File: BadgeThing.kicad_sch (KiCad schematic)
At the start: 62 parts, among them J2 Ext 5V, J3 External 3V3, J4 SWD Header, J5 USB_C_Receptacle_USB2.0, J6 Connector_Generic_Conn_01x02, J7 Conn_01x06, SW1 ESP RESET, SW2 Left, SW3 Down, SW4 Select, SW5 Up, SW6 Right, SW7 BOOTSEL, U1 ESP-12F, U3 RP2040, U4 NCP1117-3.3_SOT223, U5 W25Q32JVSS, U6 USBLC6-2SC6, Y1 12.000MHz

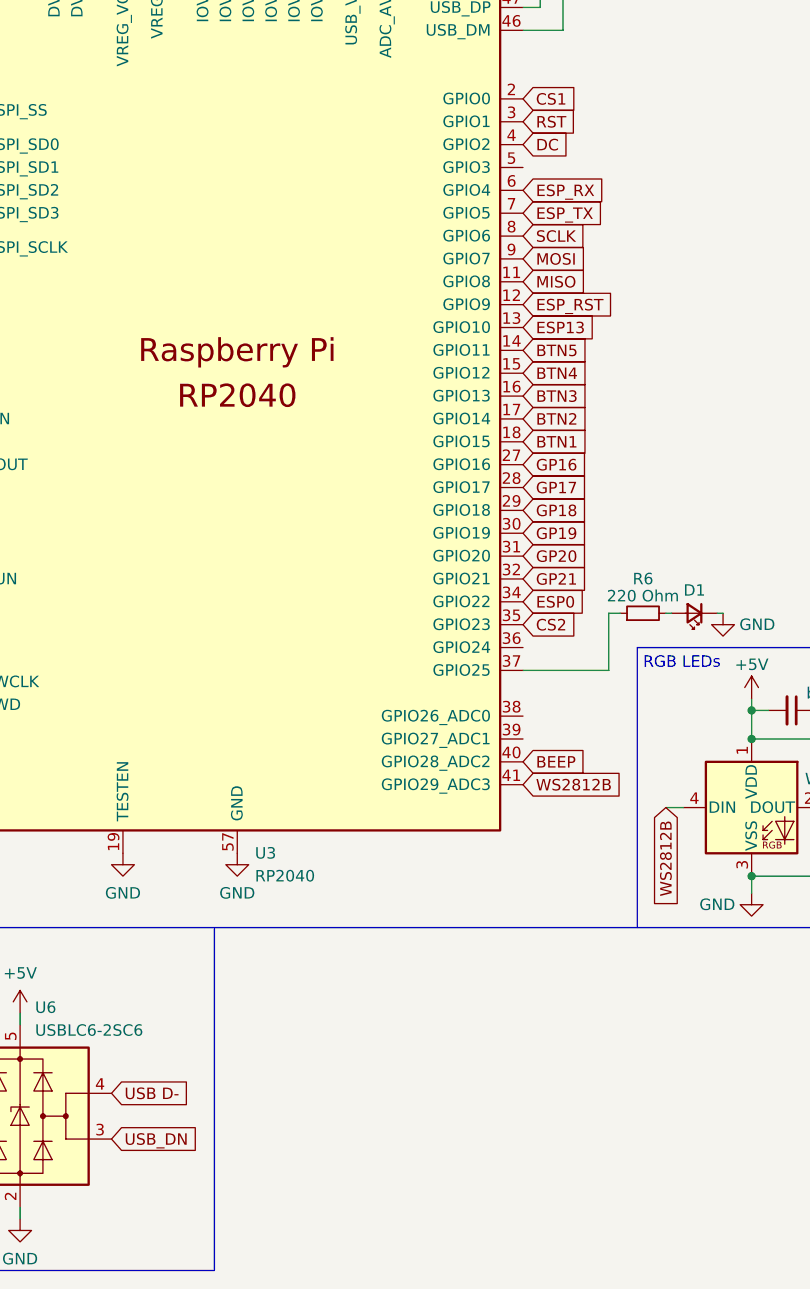
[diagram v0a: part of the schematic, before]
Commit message: Actual final real finishing touches (+test pads)
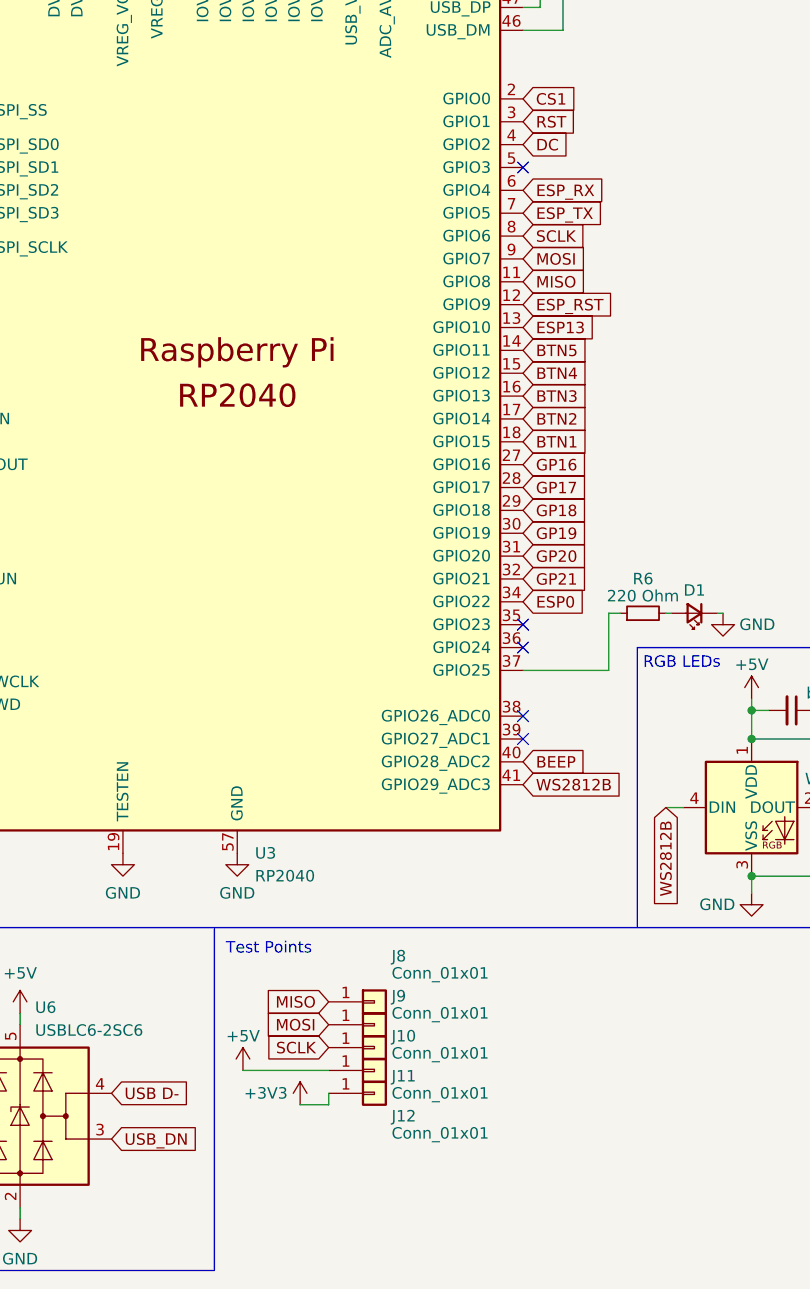
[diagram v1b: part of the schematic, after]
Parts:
- added J10, J11, J12, J8, J9: Conn_01x01, Connector_PinHeader_2.00mm:PinHeader_1x01_P2.00mm_Vertical, symbol Connector_Generic:Conn_01x01
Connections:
- net +3V3: now also J12.1 (Pin_1)
- net +5V: now also J11.1 (Pin_1)
- net MISO: now also J8.1 (Pin_1)
- net MOSI: now also J9.1 (Pin_1)
- net SCLK: now also J10.1 (Pin_1)
- net CS2: no longer names the net of U3.35 (GPIO23)
- no-connect marks 24 -> 29
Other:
- note added: "Test Points"
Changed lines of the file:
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@@
   (no_connect (at 269.875 100.33))
   (no_connect (at 55.88 139.065))
+  (no_connect (at 153.67 127))
   (no_connect (at 45.085 83.82))
   (no_connect (at 55.88 133.985))
@@
   (no_connect (at 55.88 128.905))
   (no_connect (at 45.085 76.2))
+  (no_connect (at 153.67 66.04))
+  (no_connect (at 153.67 129.54))
+  (no_connect (at 153.67 119.38))
+  (no_connect (at 153.67 116.84))
   (wire (pts (xy 45.085 45.72) (xy 43.815 45.72))
     (stroke (width 0) (type default))
@@
     (stroke (width 0) (type default))
   )
+  (wire (pts (xy 132.08 170.18) (xy 128.905 170.18))
+    (stroke (width 0) (type default))
+  )
   (wire (pts (xy 194.31 43.18) (xy 198.12 43.18))
     (stroke (width 0) (type default))
@@
     (stroke (width 0) (type default))
   )
+  (wire (pts (xy 122.555 166.37) (xy 132.08 166.37))
+    (stroke (width 0) (type default))
+  )
   (wire (pts (xy 155.575 38.1) (xy 155.575 31.75))
     (stroke (width 0) (type default))
@@
     (stroke (width 0) (type default))
   )
+  (wire (pts (xy 132.08 168.91) (xy 132.08 170.18))
+    (stroke (width 0) (type default))
+  )
   (wire (pts (xy 43.815 60.96) (xy 43.815 63.5))
     (stroke (width 0) (type default))
@@
     (effects (font (size 1.27 1.27)) (justify left bottom))
   )
+  (text "Test Points" (at 120.65 153.67 0)
+    (effects (font (size 1.27 1.27)) (justify left bottom))
+  )
   (text "Voltage Regulator" (at 193.802 64.2874 0)
     (effects (font (size 1.27 1.27)) (justify left bottom))
@@
     )
   )
+  (global_label "SCLK" (shape input) (at 132.08 163.83 180) (fields_autoplaced)
+    (effects (font (size 1.27 1.27)) (justify right))
+    (property "Intersheetrefs" "${INTERSHEET_REFS}" (at 124.3966 163.83 0)
+      (effects (font (size 1.27 1.27)) (justify right) hide)
+    )
+  )
   (global_label "SCLK" (shape input) (at 26.035 66.04 180) (fields_autoplaced)
     (effects (font (size 1.27 1.27)) (justify right))
@@
     )
   )
+  (global_label "MOSI" (shape input) (at 132.08 161.29 180) (fields_autoplaced)
+    (effects (font (size 1.27 1.27)) (justify right))
+    (property "Intersheetrefs" "${INTERSHEET_REFS}" (at 124.578 161.29 0)
+      (effects (font (size 1.27 1.27)) (justify right) hide)
+    )
+  )
   (global_label "ESP_TX" (shape input) (at 69.215 145.415 180) (fields_autoplaced)
     (effects (font (size 1.27 1.27)) (justify right))
@@
     )
   )
-  (global_label "CS2" (shape input) (at 153.67 116.84 0) (fields_autoplaced)
-    (effects (font (size 1.27 1.27)) (justify left))
-    (property "Intersheetrefs" "${INTERSHEET_REFS}" (at 160.2648 116.84 0)
-      (effects (font (size 1.27 1.27)) (justify left) hide)
-    )
-  )
   (global_label "BEEP" (shape input) (at 273.685 125.095 180) (fields_autoplaced)
     (effects (font (size 1.27 1.27)) (justify right))
@@
     )
   )
+  (global_label "MISO" (shape input) (at 132.08 158.75 180) (fields_autoplaced)
+    (effects (font (size 1.27 1.27)) (justify right))
+    (property "Intersheetrefs" "${INTERSHEET_REFS}" (at 124.578 158.75 0)
+      (effects (font (size 1.27 1.27)) (justify right) hide)
+    )
+  )
   (global_label "GP20" (shape input) (at 153.67 109.22 0) (fields_autoplaced)
     (effects (font (size 1.27 1.27)) (justify left))
@@
     )
   )
+  (symbol (lib_id "Connector_Generic:Conn_01x01") (at 137.16 158.75 0) (unit 1)
+    (in_bom yes) (on_board yes) (dnp no)
+    (property "Reference" "J8" (at 139.065 153.67 0)
+      (effects (font (size 1.27 1.27)) (justify left))
+    )
+    (property "Value" "Conn_01x01" (at 139.065 155.575 0)
+      (effects (font (size 1.27 1.27)) (justify left))
+    )
+    (property "Footprint" "Connector_PinHeader_2.00mm:PinHeader_1x01_P2.00mm_Vertical" (at 137.16 158.75 0)
+      (effects (font (size 1.27 1.27)) hide)
+    )
+    (property "Datasheet" "~" (at 137.16 158.75 0)
+      (effects (font (size 1.27 1.27)) hide)
+    )
+    (pin "1")
+    (instances
+      (project "BadgeThing"
+        (path "/35d5f6bf-e39e-48ab-813a-17587fce37db"
+          (reference "J8") (unit 1)
+        )
+      )
+    )
+  )
   (symbol (lib_id "power:GND") (at 40.64 146.685 0) (unit 1)
     (in_bom yes) (on_board yes) (dnp no)
@@
     )
   )
+  (symbol (lib_id "power:+3V3") (at 128.905 170.18 0) (unit 1)
+    (in_bom yes) (on_board yes) (dnp no)
+    (property "Reference" "#PWR047" (at 128.905 173.99 0)
+      (effects (font (size 1.27 1.27)) hide)
+    )
+    (property "Value" "+3V3" (at 125.095 168.91 0)
+      (effects (font (size 1.27 1.27)))
+    )
+    (property "Footprint" "" (at 128.905 170.18 0)
+      (effects (font (size 1.27 1.27)) hide)
+    )
+    (property "Datasheet" "" (at 128.905 170.18 0)
+      (effects (font (size 1.27 1.27)) hide)
+    )
+    (pin "1")
+    (instances
+      (project "BadgeThing"
+        (path "/35d5f6bf-e39e-48ab-813a-17587fce37db"
+          (reference "#PWR047") (unit 1)
+        )
+      )
+    )
+  )
+  (symbol (lib_id "Connector_Generic:Conn_01x01") (at 137.16 166.37 0) (unit 1)
+    (in_bom yes) (on_board yes) (dnp no)
+    (property "Reference" "J11" (at 139.065 167.005 0)
+      (effects (font (size 1.27 1.27)) (justify left))
+    )
+    (property "Value" "Conn_01x01" (at 139.065 168.91 0)
+      (effects (font (size 1.27 1.27)) (justify left))
+    )
+    (property "Footprint" "Connector_PinHeader_2.00mm:PinHeader_1x01_P2.00mm_Vertical" (at 137.16 166.37 0)
+      (effects (font (size 1.27 1.27)) hide)
+    )
+    (property "Datasheet" "~" (at 137.16 166.37 0)
+      (effects (font (size 1.27 1.27)) hide)
+    )
+    (pin "1")
+    (instances
+      (project "BadgeThing"
+        (path "/35d5f6bf-e39e-48ab-813a-17587fce37db"
+          (reference "J11") (unit 1)
+        )
+      )
+    )
+  )
   (symbol (lib_id "Device:C_Small") (at 193.04 21.59 0) (unit 1)
     (in_bom yes) (on_board yes) (dnp no)
@@
     )
   )
+  (symbol (lib_id "Connector_Generic:Conn_01x01") (at 137.16 161.29 0) (unit 1)
+    (in_bom yes) (on_board yes) (dnp no)
+    (property "Reference" "J9" (at 139.065 158.115 0)
+      (effects (font (size 1.27 1.27)) (justify left))
+    )
+    (property "Value" "Conn_01x01" (at 139.065 160.02 0)
+      (effects (font (size 1.27 1.27)) (justify left))
+    )
+    (property "Footprint" "Connector_PinHeader_2.00mm:PinHeader_1x01_P2.00mm_Vertical" (at 137.16 161.29 0)
+      (effects (font (size 1.27 1.27)) hide)
+    )
+    (property "Datasheet" "~" (at 137.16 161.29 0)
+      (effects (font (size 1.27 1.27)) hide)
+    )
+    (pin "1")
+    (instances
+      (project "BadgeThing"
+        (path "/35d5f6bf-e39e-48ab-813a-17587fce37db"
+          (reference "J9") (unit 1)
+        )
+      )
+    )
+  )
   (symbol (lib_id "Switch:SW_Push") (at 69.215 161.29 0) (unit 1)
     (in_bom yes) (on_board yes) (dnp no)
@@
     )
   )
+  (symbol (lib_id "Connector_Generic:Conn_01x01") (at 137.16 163.83 0) (unit 1)
+    (in_bom yes) (on_board yes) (dnp no)
+    (property "Reference" "J10" (at 139.065 162.56 0)
+      (effects (font (size 1.27 1.27)) (justify left))
+    )
+    (property "Value" "Conn_01x01" (at 139.065 164.465 0)
+      (effects (font (size 1.27 1.27)) (justify left))
+    )
+    (property "Footprint" "Connector_PinHeader_2.00mm:PinHeader_1x01_P2.00mm_Vertical" (at 137.16 163.83 0)
+      (effects (font (size 1.27 1.27)) hide)
+    )
+    (property "Datasheet" "~" (at 137.16 163.83 0)
+      (effects (font (size 1.27 1.27)) hide)
+    )
+    (pin "1")
+    (instances
+      (project "BadgeThing"
+        (path "/35d5f6bf-e39e-48ab-813a-17587fce37db"
+          (reference "J10") (unit 1)
+        )
+      )
+    )
+  )
   (symbol (lib_id "power:GND") (at 41.91 19.05 0) (unit 1)
     (in_bom yes) (on_board yes) (dnp no)
@@
     )
   )
+  (symbol (lib_id "Connector_Generic:Conn_01x01") (at 137.16 168.91 0) (unit 1)
+    (in_bom yes) (on_board yes) (dnp no)
+    (property "Reference" "J12" (at 139.065 171.45 0)
+      (effects (font (size 1.27 1.27)) (justify left))
+    )
+    (property "Value" "Conn_01x01" (at 139.065 173.355 0)
+      (effects (font (size 1.27 1.27)) (justify left))
+    )
+    (property "Footprint" "Connector_PinHeader_2.00mm:PinHeader_1x01_P2.00mm_Vertical" (at 137.16 168.91 0)
+      (effects (font (size 1.27 1.27)) hide)
+    )
+    (property "Datasheet" "~" (at 137.16 168.91 0)
+      (effects (font (size 1.27 1.27)) hide)
+    )
+    (pin "1")
+    (instances
+      (project "BadgeThing"
+        (path "/35d5f6bf-e39e-48ab-813a-17587fce37db"
+          (reference "J12") (unit 1)
+        )
+      )
+    )
+  )
   (symbol (lib_id "Switch:SW_Push") (at 33.02 161.29 0) (unit 1)
     (in_bom yes) (on_board yes) (dnp no)
@@
         )
       )
+    )
+  )
+  (symbol (lib_name "+5V_3") (lib_id "power:+5V") (at 122.555 166.37 0) (unit 1)
+    (in_bom yes) (on_board yes) (dnp no) (fields_autoplaced)
+    (property "Reference" "#PWR046" (at 122.555 170.18 0)
+      (effects (font (size 1.27 1.27)) hide)
+    )
+    (property "Value" "+5V" (at 122.555 162.56 0)
+      (effects (font (size 1.27 1.27)))
+    )
+    (property "Footprint" "" (at 122.555 166.37 0)
+      (effects (font (size 1.27 1.27)) hide)
+    )
+    (property "Datasheet" "" (at 122.555 166.37 0)
+      (effects (font (size 1.27 1.27)) hide)
+    )
+    (pin "1")
+    (instances
+      (project "BadgeThing"
+        (path "/35d5f6bf-e39e-48ab-813a-17587fce37db"
+          (reference "#PWR046") (unit 1)
+        )
+      )
